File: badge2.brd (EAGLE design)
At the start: 41.6 x 108 mm, 79 parts, among them IC1 ESP32-PICO-D4, Q1 CJ2302, Q2 CJ2302, Q3 FDN340P, Q4 CJ2302, U2 STM32F103CBT6, U3 MCP73831, Y1 8MHz

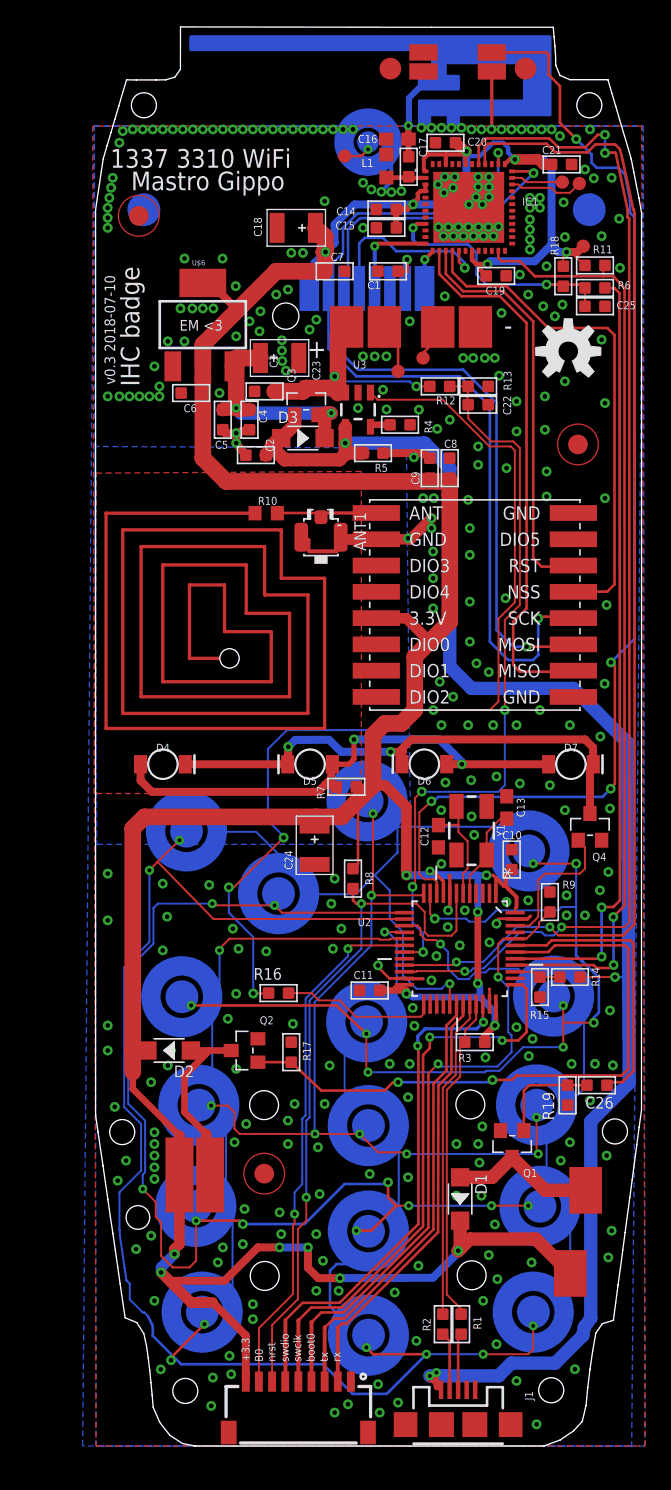
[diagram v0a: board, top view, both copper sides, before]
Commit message: Added license
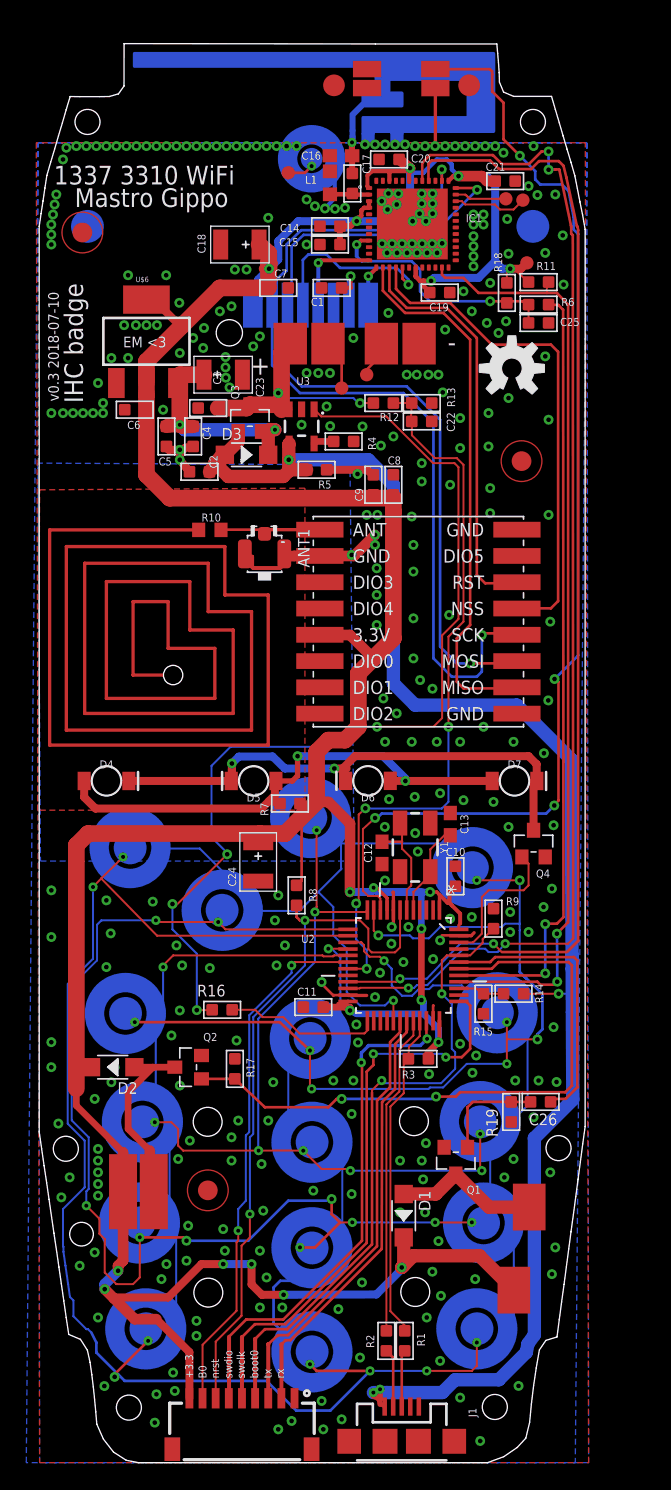
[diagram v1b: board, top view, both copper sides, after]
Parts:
- removed U$5: (no value), SparkFun-Aesthetics:OSHW-LOGO-M
- added LOGO1: OSHW-LOGOM, SparkFun-Aesthetics:OSHW-LOGO-M
- R3: value 2K -> 1.5K
- moved R13 4.48 mm to (29.1, 80.6)
- moved D1 4.48 mm to (27.7, 18.8)
- moved R1 4.48 mm to (27.8, 9.27)
- moved ANT1 4.48 mm to (17.1, 69.2)
- moved C15 4.48 mm to (22.1, 92.7)
- moved C16 4.48 mm to (23.0, 99.5)
- moved C17 4.48 mm to (23.8, 97.4)
- moved C18 4.48 mm to (15.3, 92.7)
- moved C22 4.48 mm to (29.1, 79.2)
- moved C3 4.48 mm to (12.9, 80.3)
- moved FID2 4.48 mm to (3.28, 93.6)
- moved FID3 4.48 mm to (36.7, 76.2)
- moved Q3 4.48 mm to (16.0, 79.5)
- moved R12 4.48 mm to (26.2, 80.6)
- moved TP5 4.48 mm to (23.0, 81.8)
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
